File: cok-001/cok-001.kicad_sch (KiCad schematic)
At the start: 21 parts, among them U6005 NCP511SN33T1G, U6006 NCP511SN18T1, U6009 NCP511SN33T1G

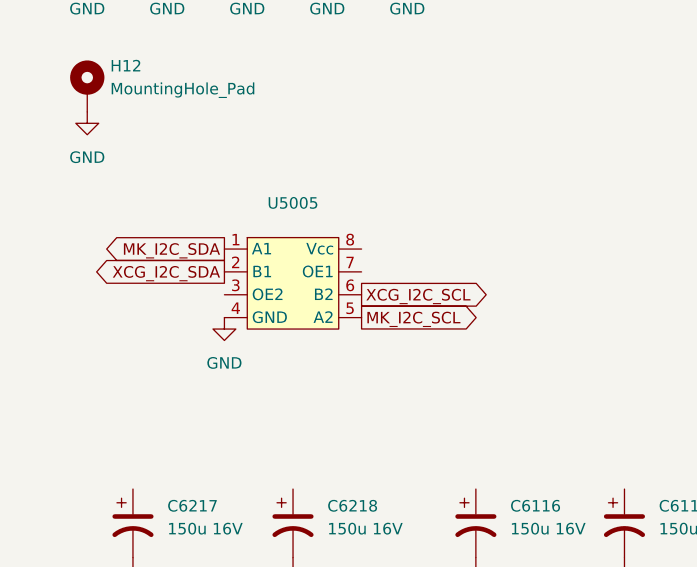
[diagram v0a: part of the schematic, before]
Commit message: footprints
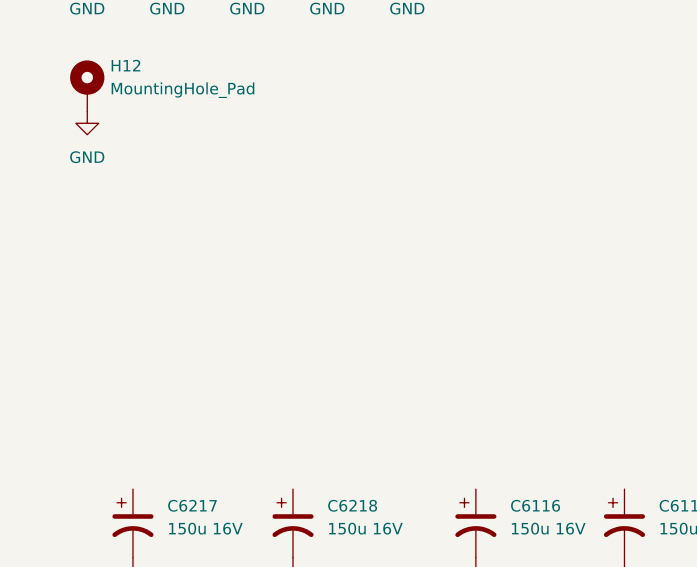
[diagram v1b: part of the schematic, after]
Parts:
- removed U5005: ~, Package_SO:VSSOP-8_2.3x2mm_P0.5mm, symbol PS3:TC7WB66FK
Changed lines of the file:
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@@
-		)
-	)
-	(global_label "XCG_I2C_SCL"
-		(shape output)
-		(at 53.34 149.86 0)
-		(fields_autoplaced yes)
-		(effects
-			(font
-				(size 1.27 1.27)
-			)
-			(justify left)
-		)
-		(property "Intersheetrefs" "${INTERSHEET_REFS}"
-			(at 68.6018 149.86 0)
-			(effects
-				(font
-					(size 1.27 1.27)
-				)
-				(justify left)
-				(hide yes)
-			)
-		)
-	)
-	(global_label "MK_I2C_SCL"
-		(shape output)
-		(at 53.34 152.4 0)
-		(fields_autoplaced yes)
-		(effects
-			(font
-				(size 1.27 1.27)
-			)
-			(justify left)
-		)
-		(property "Intersheetrefs" "${INTERSHEET_REFS}"
-			(at 67.5737 152.4 0)
-			(effects
-				(font
-					(size 1.27 1.27)
-				)
-				(justify left)
-				(hide yes)
-			)
-		)
-	)
-	(global_label "XCG_I2C_SDA"
-		(shape output)
-		(at 38.1 147.32 180)
-		(fields_autoplaced yes)
-		(effects
-			(font
-				(size 1.27 1.27)
-			)
-			(justify right)
-		)
-		(property "Intersheetrefs" "${INTERSHEET_REFS}"
-			(at 22.7777 147.32 0)
-			(effects
-				(font
-					(size 1.27 1.27)
-				)
-				(justify right)
-				(hide yes)
-			)
-		)
-	)
-	(global_label "MK_I2C_SDA"
-		(shape output)
-		(at 38.1 144.78 180)
-		(fields_autoplaced yes)
-		(effects
-			(font
-				(size 1.27 1.27)
-			)
-			(justify right)
-		)
-		(property "Intersheetrefs" "${INTERSHEET_REFS}"
-			(at 23.8058 144.78 0)
-			(effects
-				(font
-					(size 1.27 1.27)
-				)
-				(justify right)
-				(hide yes)
-			)
 		)
 	)
@@
 	)
 	(symbol
-		(lib_id "power:GND")
-		(at 38.1 152.4 0)
-		(unit 1)
-		(exclude_from_sim no)
-		(in_bom yes)
-		(on_board yes)
-		(dnp no)
-		(fields_autoplaced yes)
-		(property "Reference" "#PWR0140"
-			(at 38.1 158.75 0)
-			(effects
-				(font
-					(size 1.27 1.27)
-				)
-				(hide yes)
-			)
-		)
-		(property "Value" "GND"
-			(at 38.1 157.48 0)
-			(effects
-				(font
-					(size 1.27 1.27)
-				)
-			)
-		)
-		(property "Footprint" ""
-			(at 38.1 152.4 0)
-			(effects
-				(font
-					(size 1.27 1.27)
-				)
-				(hide yes)
-			)
-		)
-		(property "Datasheet" ""
-			(at 38.1 152.4 0)
-			(effects
-				(font
-					(size 1.27 1.27)
-				)
-				(hide yes)
-			)
-		)
-		(property "Description" "Power symbol creates a global label with name \"GND\" , ground"
-			(at 38.1 152.4 0)
-			(effects
-				(font
-					(size 1.27 1.27)
-				)
-				(hide yes)
-			)
-		)
-		(pin "1"
-		)
-		(instances
-			(project "cok-001"
-				(path "/976eb78d-8215-4cc0-9d72-f9d535c7970b"
-					(reference "#PWR0140")
-					(unit 1)
-				)
-			)
-		)
-	)
-	(symbol
 		(lib_id "Regulator_Linear:MIC5219-3.3YM5")
 		(at 306.07 177.8 0)
@@
 				(path "/976eb78d-8215-4cc0-9d72-f9d535c7970b"
 					(reference "#PWR0178")
-					(unit 1)
-				)
-			)
-		)
-	)
-	(symbol
-		(lib_id "PS3:TC7WB66FK")
-		(at 45.72 142.24 0)
-		(unit 1)
-		(exclude_from_sim no)
-		(in_bom yes)
-		(on_board yes)
-		(dnp no)
-		(fields_autoplaced yes)
-		(property "Reference" "U5005"
-			(at 45.72 139.7 0)
-			(effects
-				(font
-					(size 1.27 1.27)
-				)
-			)
-		)
-		(property "Value" "~"
-			(at 45.72 142.24 0)
-			(effects
-				(font
-					(size 1.27 1.27)
-				)
-			)
-		)
-		(property "Footprint" "Package_SO:VSSOP-8_2.3x2mm_P0.5mm"
-			(at 45.72 142.24 0)
-			(effects
-				(font
-					(size 1.27 1.27)
-				)
-				(hide yes)
-			)
-		)
-		(property "Datasheet" ""
-			(at 45.72 142.24 0)
-			(effects
-				(font
-					(size 1.27 1.27)
-				)
-				(hide yes)
-			)
-		)
-		(property "Description" ""
-			(at 45.72 142.24 0)
-			(effects
-				(font
-					(size 1.27 1.27)
-				)
-				(hide yes)
-			)
-		)
-		(pin "3"
-		)
-		(pin "2"
-		)
-		(pin "1"
-		)
-		(pin "7"
-		)
-		(pin "4"
-		)
-		(pin "5"
-		)
-		(pin "6"
-		)
-		(pin "8"
-		)
-		(instances
-			(project ""
-				(path "/976eb78d-8215-4cc0-9d72-f9d535c7970b"
-					(reference "U5005")
 					(unit 1)
 				)
@@
 			(project "cok-001"
 				(path "/976eb78d-8215-4cc0-9d72-f9d535c7970b"
-					(page "20")
-				)
-			)
+					(page "50")
+				)
+			)
